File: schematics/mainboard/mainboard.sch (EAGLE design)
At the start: 119 parts, among them IC1 OPA2344P, IC2 LM339N, IC3 74AHC00D, IC5 LM2576-5.0, IC6 LM2576-3.3, Q1 BD140, Q2 BD140, Q3 IRF540, T3 BC847, T4 BC847, T5 BC847, T6 BC847, T7 BC847, T8 BC847, U1 STM32F777VIT

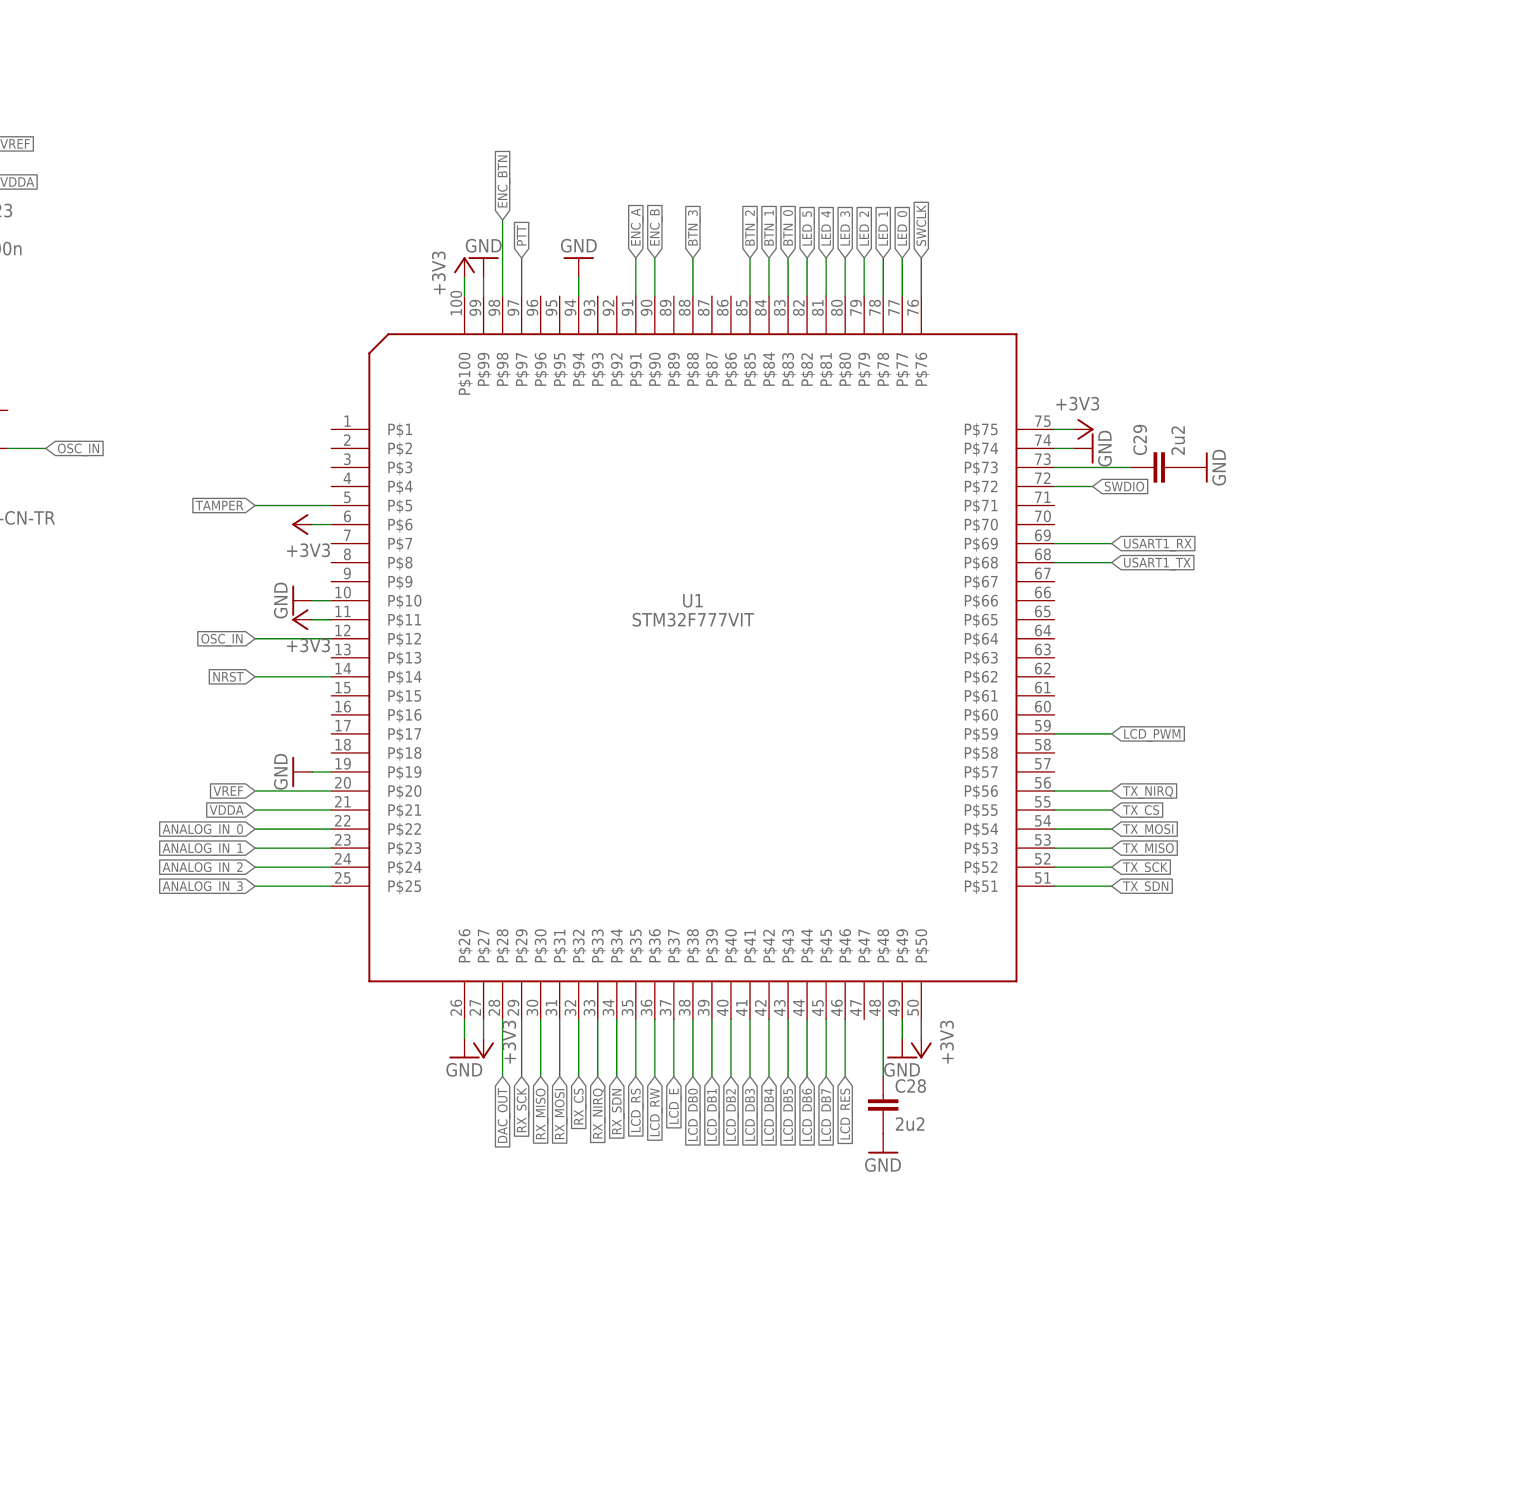
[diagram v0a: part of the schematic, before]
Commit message: Add files via upload
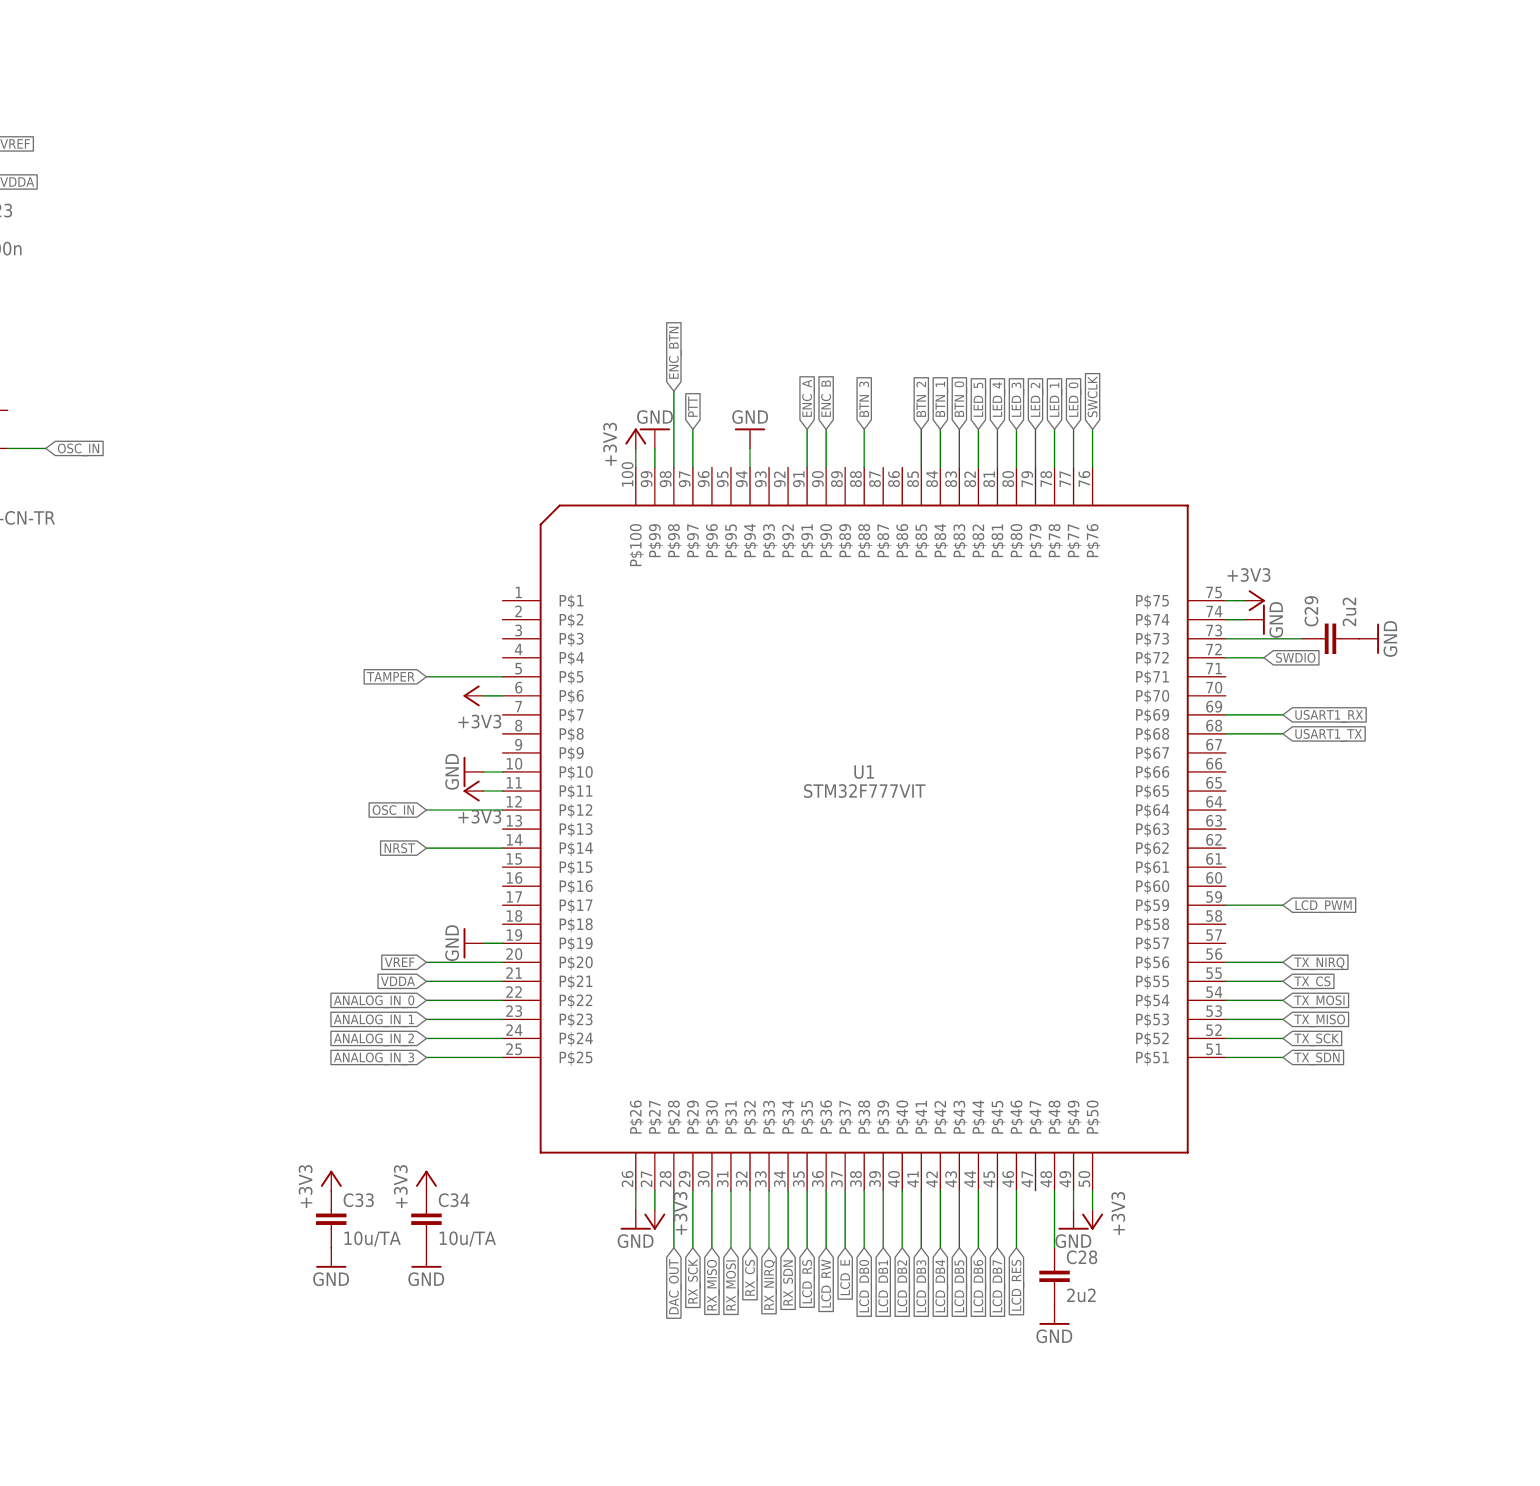
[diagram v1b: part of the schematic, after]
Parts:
- added C33, C34: 10u/TA, resistor:C-EUC1206
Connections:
- net +3V3: now also C33.1, C34.1
- net GND: now also C33.2, C34.2
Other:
- moved on the sheet: C28, C29, U1
